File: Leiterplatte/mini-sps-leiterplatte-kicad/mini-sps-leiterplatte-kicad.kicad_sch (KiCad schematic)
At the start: 42 parts, among them J1 Screw_Terminal_01x03, J2 Screw_Terminal_01x03, J3 Screw_Terminal_01x03, J4 Screw_Terminal_01x03, J5 Screw_Terminal_01x02, J6 Screw_Terminal_01x03, J7 Screw_Terminal_01x02, K1 SRD-05VDC-SL-C, K2 SRD-05VDC-SL-C, K3 SRD-05VDC-SL-C, U1 L7805

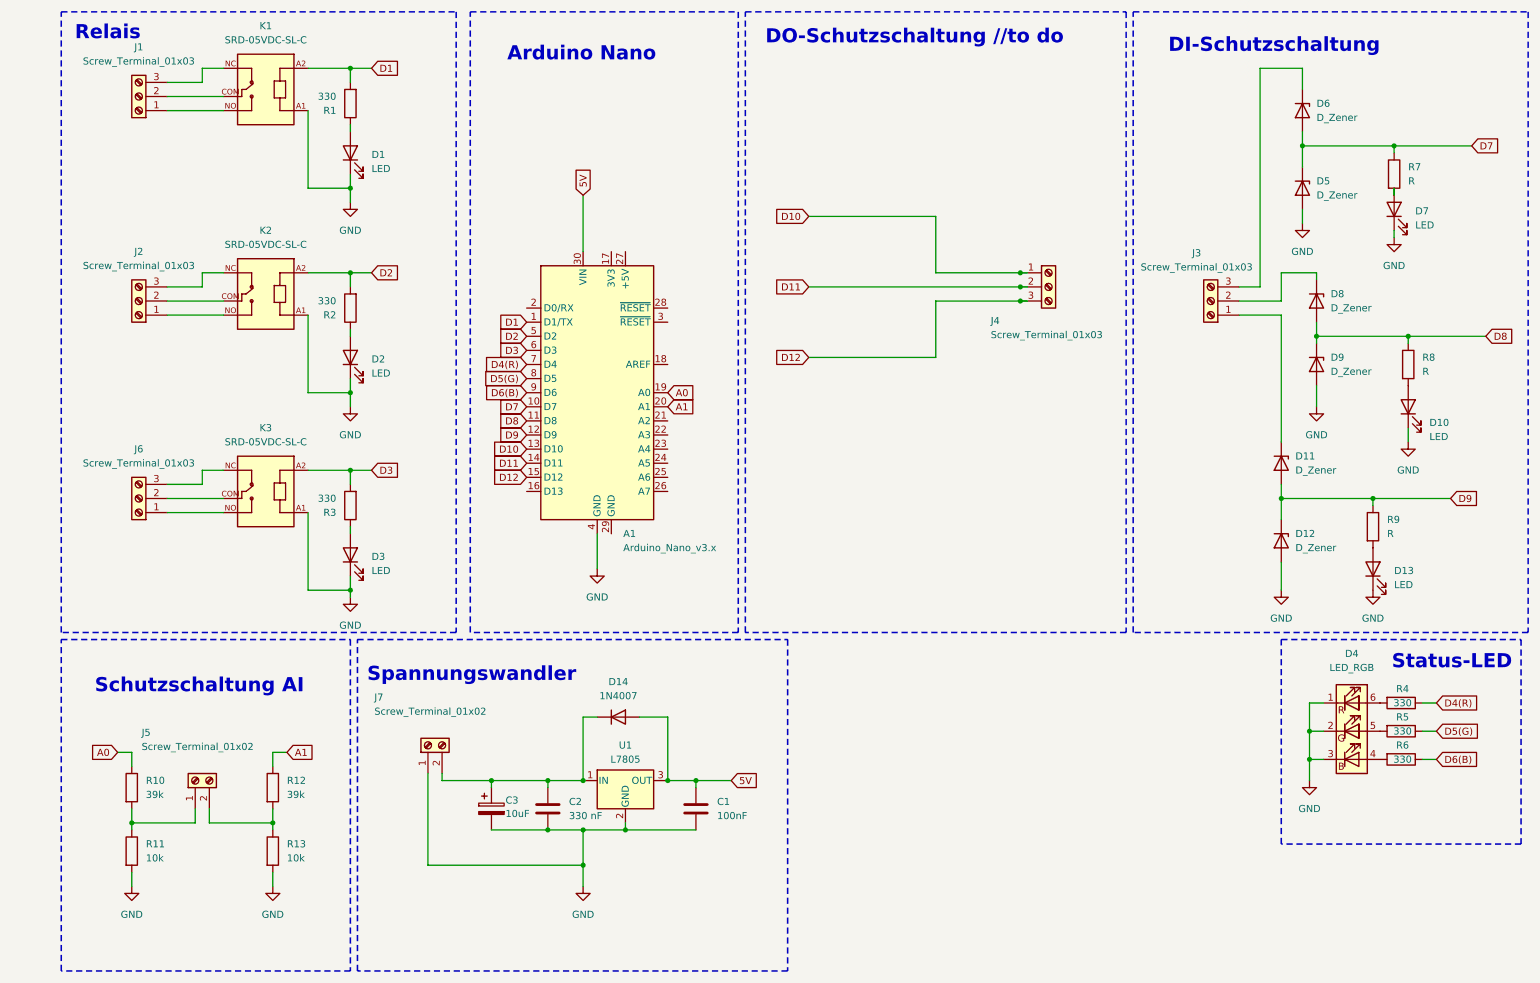
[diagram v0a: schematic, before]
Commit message: alles auf den neusten fucking stand
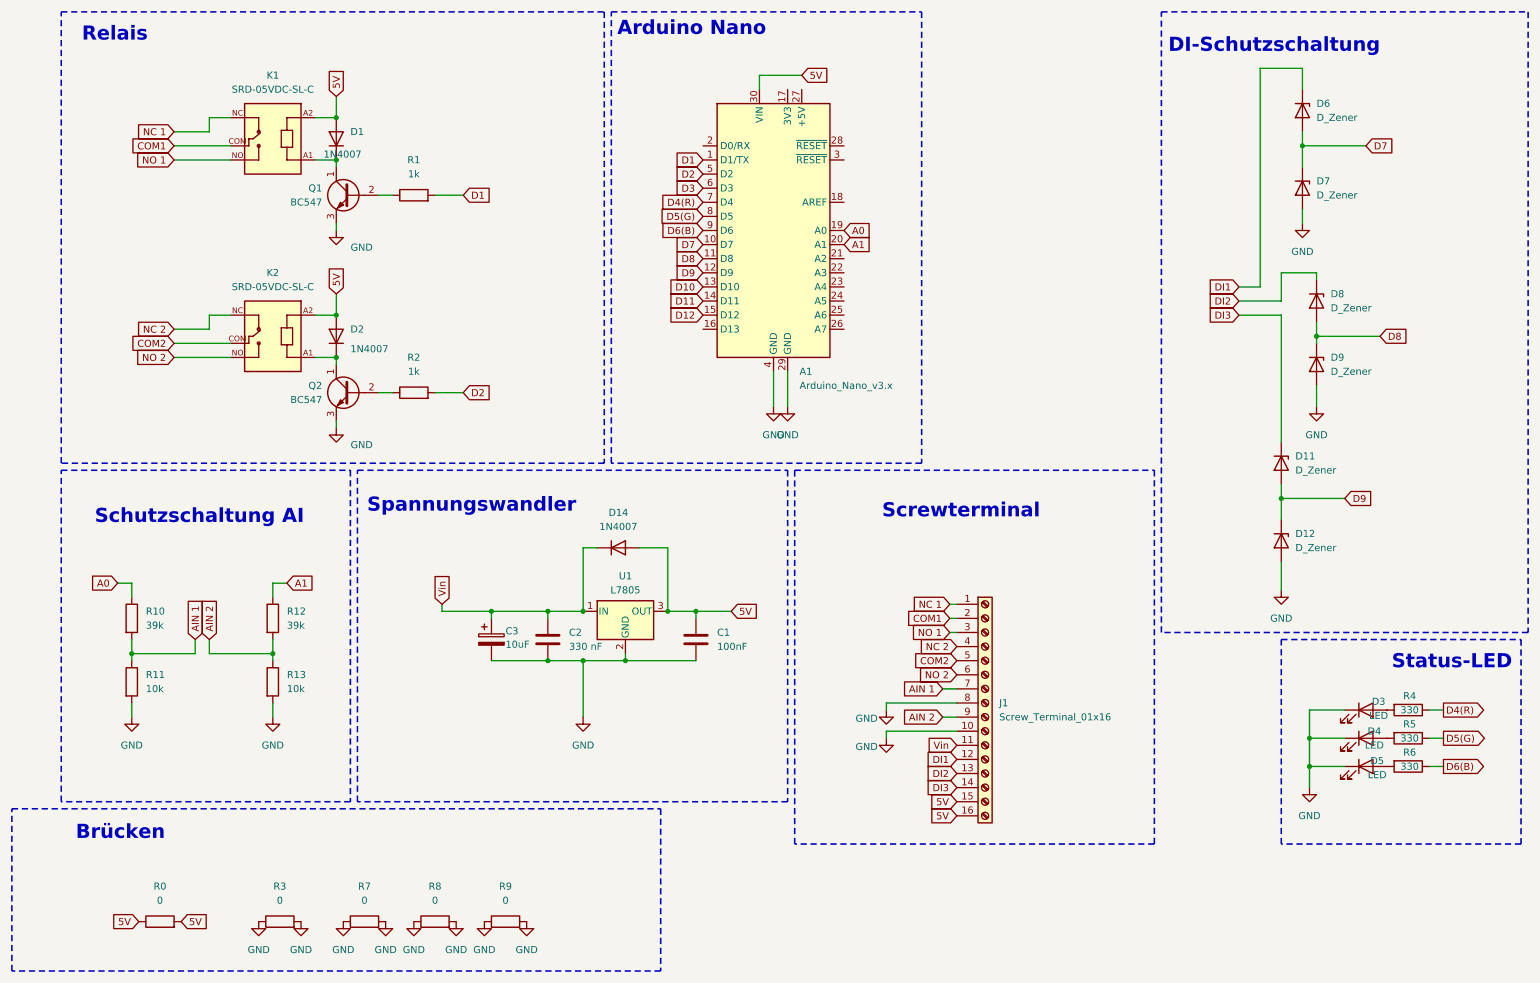
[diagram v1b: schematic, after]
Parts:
- removed D1, D10, D13, D2, D7: LED, LED_THT:LED_D5.0mm, symbol Device:LED
- removed D4: LED_RGB, LED_THT:LED_D5.0mm-4_RGB_Wide_Pins, symbol Device:LED_RGB
- removed J1, J2, J3, J4, J6: Screw_Terminal_01x03, TerminalBlock:TerminalBlock_bornier-3_P5.08mm, symbol Connector:Screw_Terminal_01x03
- removed J5, J7: Screw_Terminal_01x02, TerminalBlock:TerminalBlock_bornier-2_P5.08mm, symbol Connector:Screw_Terminal_01x02
- removed K3: SRD-05VDC-SL-C, custom:RELAY_SRD-05VDC-SL-C, symbol custom:SRD-05VDC-SL-C
- added D1, D2: 1N4007, Diode_THT:D_DO-15_P15.24mm_Horizontal, symbol Device:D
- added D4, D5: LED, LED_THT:LED_D5.0mm, symbol Device:LED
- added J1: Screw_Terminal_01x16, TerminalBlock_CUI:TerminalBlock_CUI_TB007-508-16_1x16_P5.08mm_Horizontal, symbol Connector:Screw_Terminal_01x16
- added Q1, Q2: BC547, Package_TO_SOT_THT:TO-92L_Inline_Wide, symbol Transistor_BJT:BC547
- added R0: 0, Resistor_THT:R_Axial_DIN0207_L6.3mm_D2.5mm_P10.16mm_Horizontal, symbol Device:R
- R1, R2: value 330 -> 1k
- R3: value 330 -> 0
- R7, R8, R9: value R -> 0
- renumbered D5 to D7
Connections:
- net 5V: now also K1.A2, K2.A2, D1.2 (A), D2.2 (A), J1.15 (Pin_15), J1.16 (Pin_16), R0.1, R0.2
- net D1: no longer K1.A2
- net D2: no longer K2.A2
- net D3: no longer R3.2
- net D7: no longer R7.1
- net D8: no longer R8.1
- net D9: no longer R9.1
- net GND: now also A1.29 (GND), R3.1, R3.2, R7.1, R7.2, R8.1, R8.2, R9.1, R9.2, D4.1 (K), D5.1 (K), J1.10 (Pin_10), J1.8 (Pin_8), Q1.3 (E), Q2.3 (E); no longer K1.A1, K2.A1
- net at R6.2: now also D5.2 (A)
- net at R5.2: now also D4.2 (A)
- net at R4.2: now also D3.2 (A)
- net AIN 1: now reaches R10.2, R11.1
- net AIN 1: now also J1.7 (Pin_7)
- net Vin: now reaches C2.1, C3.1, D14.1 (K), U1.1 (IN)
- net Vin: now also J1.11 (Pin_11)
- net AIN 2: now reaches R12.2, R13.1
- net AIN 2: now also J1.9 (Pin_9)
- net DI3: now reaches D11.1 (K)
- net DI3: now also J1.14 (Pin_14)
- net DI1: now reaches D6.1 (K)
- net DI1: now also J1.12 (Pin_12)
- net NO 1: now reaches K1.NO
- net NO 1: now also J1.3 (Pin_3)
- net COM1: now reaches K1.COM
- net COM1: now also J1.2 (Pin_2)
- net NC 1: now reaches K1.NC
- net NC 1: now also J1.1 (Pin_1)
- net DI2: now reaches D8.1 (K)
- net DI2: now also J1.13 (Pin_13)
- net at R1.1: now also Q1.2 (B)
- net at R2.1: now also Q2.2 (B)
- net COM2: now reaches K2.COM
- net COM2: now also J1.5 (Pin_5)
- net NC 2: now reaches K2.NC
- net NC 2: now also J1.4 (Pin_4)
- net NO 2: now reaches K2.NO
- net NO 2: now also J1.6 (Pin_6)
- new net: D2.1 (K), K2.A1, Q2.1 (C)
- new net: D1.1 (K), K1.A1, Q1.1 (C)
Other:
- note added: "Brücken"
- note added: "Screwterminal"
- note removed: "DO-Schutzschaltung //to do"
- moved on the sheet: A1, C1, C2, C3, D14, K1, R10, R11, R12, R13, R4, R5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
